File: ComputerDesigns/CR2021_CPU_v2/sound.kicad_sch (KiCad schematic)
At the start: 5 parts, among them U1 LM324

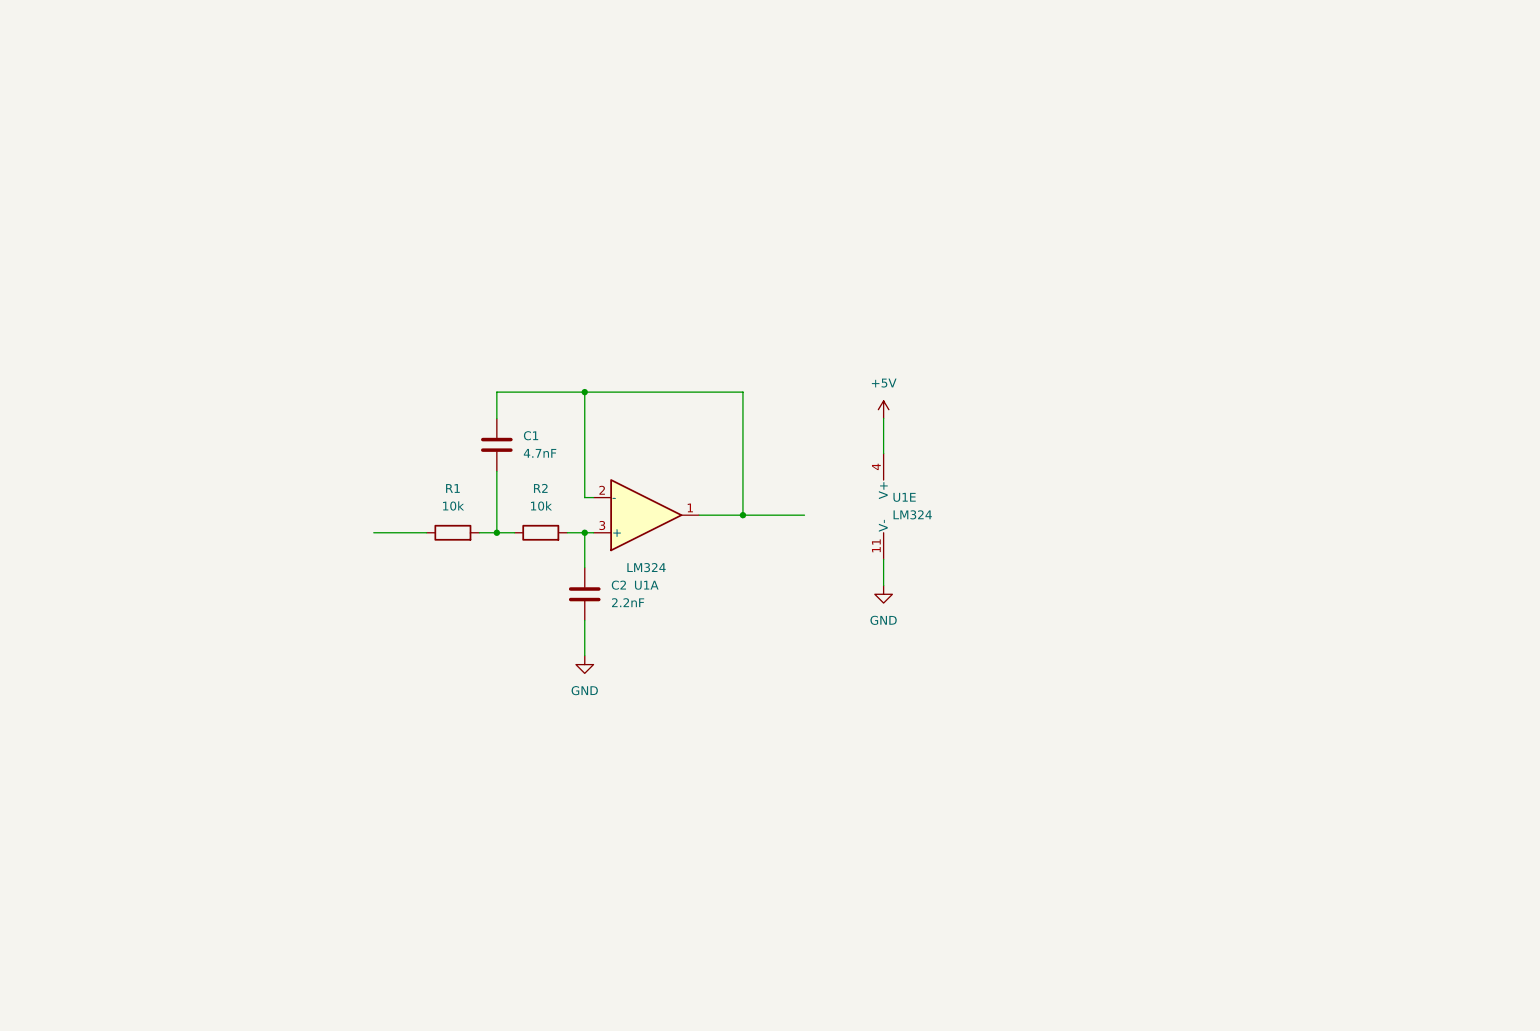
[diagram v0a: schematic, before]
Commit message: add sound
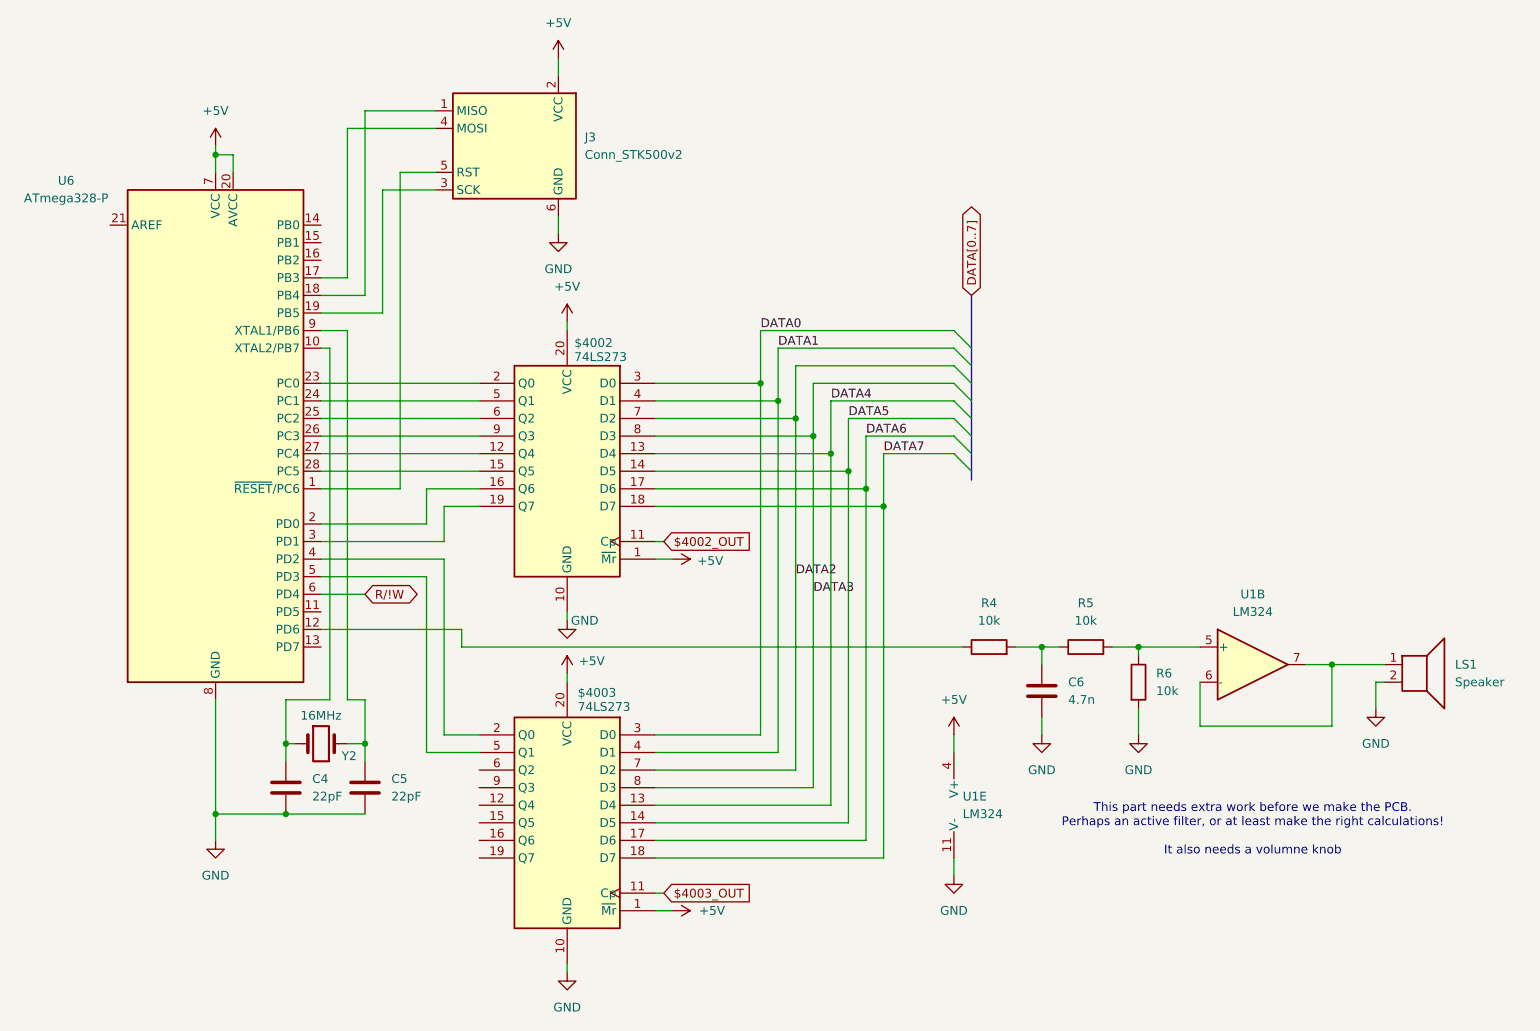
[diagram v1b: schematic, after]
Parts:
- removed C1: 4.7nF, symbol Device:C
- removed C2: 2.2nF, symbol Device:C
- removed R1, R2: 10k, symbol Device:R
- removed unit 1 of U1
- added $4002, $4003: 74LS273, Package_DIP:DIP-20_W7.62mm, symbol 74xx:74LS273
- added C4, C5: 22pF, symbol Device:C
- added C6: 4.7n, symbol Device:C
- added J3: Conn_STK500v2, Connector_IDC:IDC-Header_2x03_P2.54mm_Vertical, symbol Custom:Conn_STK500v2
- added LS1: Speaker, Connector_PinHeader_2.54mm:PinHeader_1x02_P2.54mm_Vertical, symbol Device:Speaker
- added R4, R5, R6: 10k, symbol Device:R
- added unit 2 of U1
- added U6: ATmega328-P, Package_DIP:DIP-28_W7.62mm, symbol MCU_Microchip_ATmega:ATmega328-P
- added Y2: 16MHz, symbol Device:Crystal
- U1: footprint (none) -> Package_DIP:DIP-14_W7.62mm
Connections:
- net +5V: now also $4002.1 (~{Mr}), $4002.20 (VCC), $4003.1 (~{Mr}), $4003.20 (VCC), J3.2 (VCC), U6.20 (AVCC), U6.7 (VCC)
- net GND: now also $4002.10 (GND), $4003.10 (GND), C4.2, C5.2, C6.2, J3.6 (GND), LS1.2, R6.2, U6.22 (GND), U6.8 (GND)
- new net: R4.1, U6.12 (PD6)
- new net: C6.1, R4.2, R5.1
- new net: C5.1, U6.9 (XTAL1/PB6), Y2.2
- new net: $4003.2 (Q0), U6.4 (PD2)
- new net: $4003.5 (Q1), U6.5 (PD3)
- new net: LS1.1, U1.6 (-), U1.7
- new net: C4.1, U6.10 (XTAL2/PB7), Y2.1
- new net: R5.2, R6.1, U1.5 (+)
- new net: $4002.12 (Q4), U6.27 (PC4)
- new net: $4002.15 (Q5), U6.28 (PC5)
- new net: $4002.16 (Q6), U6.2 (PD0)
- new net: $4002.19 (Q7), U6.3 (PD1)
- new net: $4002.2 (Q0), U6.23 (PC0)
- new net: $4002.5 (Q1), U6.24 (PC1)
- new net: $4002.6 (Q2), U6.25 (PC2)
- new net: $4002.9 (Q3), U6.26 (PC3)
- new net: J3.5 (RST), U6.1 (~{RESET}/PC6)
- new net: J3.4 (MOSI), U6.17 (PB3)
- new net: J3.1 (MISO), U6.18 (PB4)
- new net: J3.3 (SCK), U6.19 (PB5)
- new net $4002_OUT: $4002.11 (Cp)
- new net $4003_OUT: $4003.11 (Cp)
- new net DATA0: $4002.3 (D0), $4003.3 (D0)
- new net DATA1: $4002.4 (D1), $4003.4 (D1)
- new net DATA2: $4002.7 (D2), $4003.7 (D2)
- new net DATA3: $4002.8 (D3), $4003.8 (D3)
- new net DATA4: $4002.13 (D4), $4003.13 (D4)
- new net DATA5: $4002.14 (D5), $4003.14 (D5)
- new net DATA6: $4002.17 (D6), $4003.17 (D6)
- new net DATA7: $4002.18 (D7), $4003.18 (D7)
- new net R/!W: U6.6 (PD4)
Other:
- note added: "This part needs extra work before we make the PCB. Perhaps an active filter, or at least make the right calculations! It also needs a volumne knob"
